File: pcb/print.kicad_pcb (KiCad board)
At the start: 2 copper layers, 12.4 x 46.4 mm, 23 parts, among them J1 USB_C_Receptacle_USB2.0_16P, J2 WS2812, SW1 Cycle, U1 FT232RL, U2 ATtiny85-20S

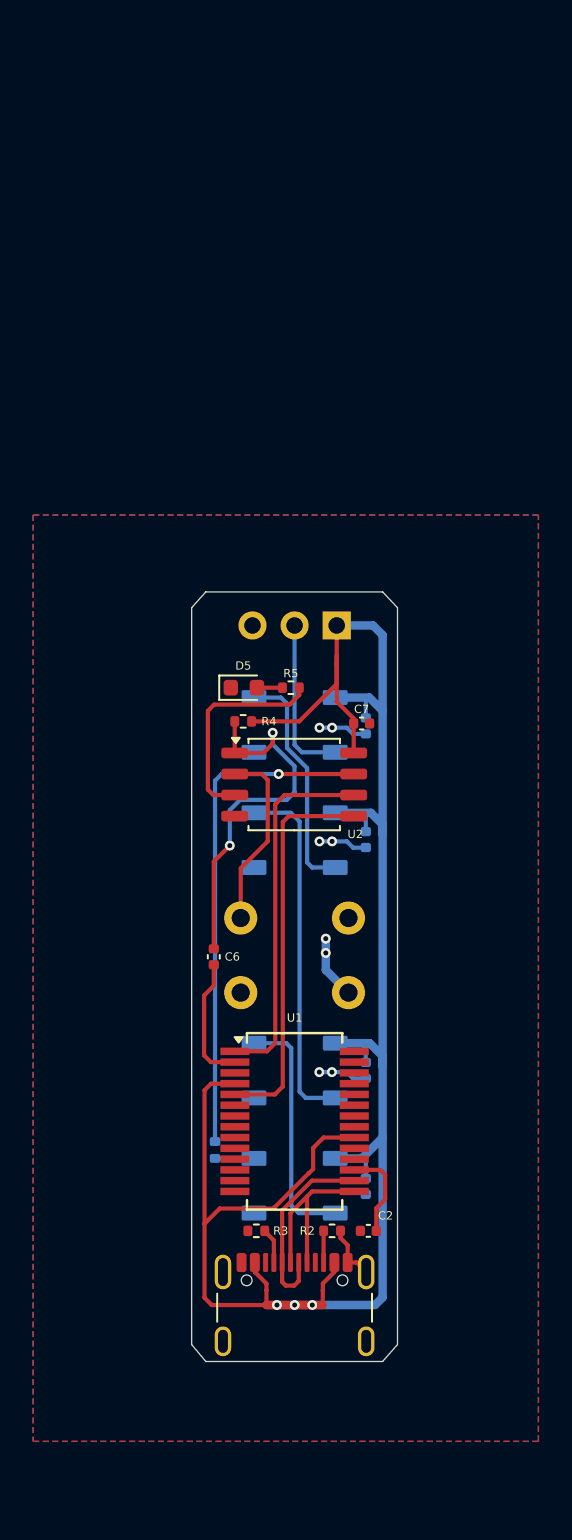
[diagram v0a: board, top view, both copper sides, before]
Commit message: pcb v1.1.0 update
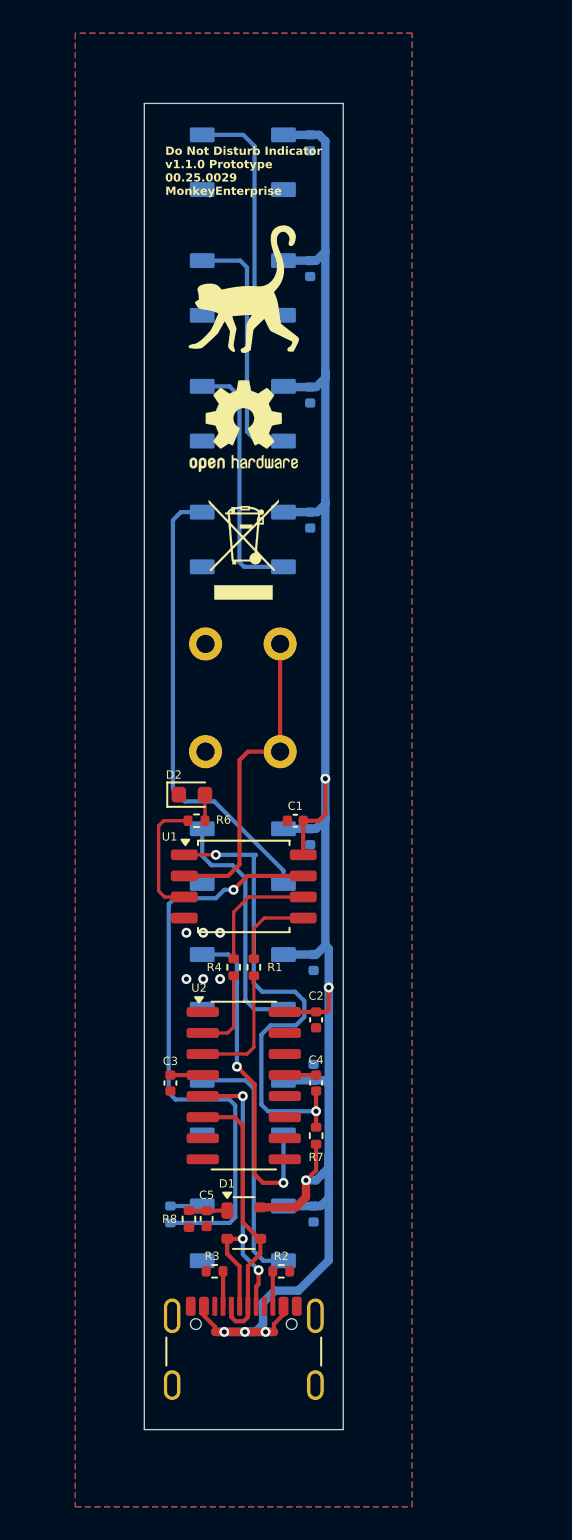
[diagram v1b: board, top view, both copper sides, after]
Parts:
- removed J2: WS2812, Connector_PinHeader_2.54mm:PinHeader_1x03_P2.54mm_Vertical
- added C10: 100nF, Capacitor_SMD:C_0402_1005Metric, B.Cu at (152.1, 74.0)
- added C11: 100nF, Capacitor_SMD:C_0402_1005Metric, B.Cu at (152.1, 66.4)
- added C12: 100nF, Capacitor_SMD:C_0402_1005Metric, B.Cu at (152.1, 58.8)
- added C13: 100nF, Capacitor_SMD:C_0402_1005Metric, B.Cu at (152.1, 51.2)
- added C8: 100nF, Capacitor_SMD:C_0402_1005Metric, B.Cu at (152.3, 100.7)
- added C9: 100nF, Capacitor_SMD:C_0402_1005Metric, B.Cu at (152.1, 93.1)
- added D10: WS2812B, Lib_WS2812B:LED_WS2812B_PLCC4_5.0x5.0mm_P3.2mm, B.Cu at (148.0, 52.4)
- added D6: WS2812B, Lib_WS2812B:LED_WS2812B_PLCC4_5.0x5.0mm_P3.2mm, B.Cu at (148.0, 94.2)
- added D7: WS2812B, Lib_WS2812B:LED_WS2812B_PLCC4_5.0x5.0mm_P3.2mm, B.Cu at (148.0, 75.1)
- added D8: WS2812B, Lib_WS2812B:LED_WS2812B_PLCC4_5.0x5.0mm_P3.2mm, B.Cu at (148.0, 67.5)
- added D9: WS2812B, Lib_WS2812B:LED_WS2812B_PLCC4_5.0x5.0mm_P3.2mm, B.Cu at (148.0, 60.0)
- added R6: 4K7, Resistor_SMD:R_0402_1005Metric, F.Cu at (145.2, 92.1)
- added R7: 10K0, Resistor_SMD:R_0402_1005Metric, F.Cu at (152.5, 111.1)
- added R8: 1M0, Resistor_SMD:R_0402_1005Metric, F.Cu at (144.8, 116.1)
- added REF**: WEEE-Logo_4.2x6mm_SilkScreen, Symbol:WEEE-Logo_4.2x6mm_SilkScreen, F.Cu at (148.1, 75.7)
- added REF**: OSHW-Logo2_7.3x6mm_SilkScreen, Symbol:OSHW-Logo2_7.3x6mm_SilkScreen, F.Cu at (148.1, 68.3)
- C1, C3, C4, G***: moved to F.Cu
- C5: value 100nF -> 4.7nF/1kV; moved to F.Cu
- C6, C7: moved to B.Cu
- D1: value WS2812B -> PRTR5V0U2X; footprint LED_SMD:LED_WS2812B_PLCC4_5.0x5.0mm_P3.2mm -> Package_TO_SOT_SMD:SOT-143; moved to F.Cu
- D2: value WS2812B -> CPU; footprint LED_SMD:LED_WS2812B_PLCC4_5.0x5.0mm_P3.2mm -> Diode_SMD:D_0603_1608Metric; moved to F.Cu
- D3, D4: footprint LED_SMD:LED_WS2812B_PLCC4_5.0x5.0mm_P3.2mm -> Lib_WS2812B:LED_WS2812B_PLCC4_5.0x5.0mm_P3.2mm
- D5: value CPU -> WS2812B; footprint Diode_SMD:D_0603_1608Metric -> Lib_WS2812B:LED_WS2812B_PLCC4_5.0x5.0mm_P3.2mm; moved to B.Cu
- R1: value 4K7 -> 1K0; moved to F.Cu
- R4: value 10K0 -> 1K0
- R5: value 4K7 -> 1K0; moved to B.Cu
- U1: value FT232RL -> ATtiny85-20S; footprint Package_SO:SSOP-28_5.3x10.2mm_P0.65mm -> Package_SO:SOIC-8_5.3x5.3mm_P1.27mm
- U2: value ATtiny85-20S -> CH340C; footprint Package_SO:SOIC-8_5.3x5.3mm_P1.27mm -> Package_SO:SOIC-16_3.9x9.9mm_P1.27mm
- moved G*** 60.7 mm to (148.1, 60.1), turned to 0 degrees
- moved R5 32.6 mm to (143.7, 115.9), turned to 90 degrees
- moved C5 31.2 mm to (145.8, 116.1)
- moved D3 23.9 mm to (148.0, 117.0)
- moved D4 23.3 mm to (148.0, 109.4)
- moved C1 22.5 mm to (151.2, 92.1), turned to 180 degrees
- moved C7 21.2 mm to (152.3, 107.3), turned to 90 degrees
- moved U2 18.4 mm to (148.1, 108.1)
- moved D2 17.8 mm to (145.0, 90.5), turned to 0 degrees
- moved D5 17.7 mm to (148.0, 101.8), turned to 180 degrees
- moved C6 16.6 mm to (152.3, 115.8), turned to -90 degrees
- moved C4 15.0 mm to (152.5, 107.9)
- moved R4 14.8 mm to (147.5, 100.9), turned to -90 degrees
- moved U1 14.5 mm to (148.1, 96.1)
- moved C2 13.1 mm to (152.5, 104.1), turned to -90 degrees
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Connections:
- C2 pad 1: +3.3V -> VBUS
- C3 pad 1: VBUS -> Net-(U2-V3)
- C4 pad 1: VBUS -> Net-(U2-~{DTR})
- C4 pad 2: GND -> /~{Reset} 
- C5 pad 1: VBUS -> Net-(D1-GND)
- C6 pad 1: Net-(U1-DTR) -> VBUS
- C6 pad 2: /~{Reset}  -> GND
- D1 pad 1: VBUS -> Net-(D1-GND)
- D1 pad 2: Net-(D1-DOUT) -> /USB_D_P
- D1 pad 3: GND -> /USB_D_N
- D1 pad 4: Net-(D1-DIN) -> VBUS
- D2 pad 1: VBUS -> GND
- D2 pad 2: Net-(D2-DOUT) -> Net-(D2-A)
- D3 pad 4: Net-(D2-DOUT) -> /LED_DATA_P
- D5 pad 1: GND -> VBUS
- D5 pad 2: Net-(D5-A) -> Net-(D5-DOUT)
- J1 pad A6: /USB_P -> /USB_D_P
- J1 pad A7: /USB_N -> /USB_D_N
- J1 pad B6: /USB_P -> /USB_D_P
- J1 pad B7: /USB_N -> /USB_D_N
- R1 pad 1: /LED_DATA_P -> Net-(U1-AREF/PB0)
- R1 pad 2: Net-(D1-DIN) -> /TX_D_P
- R4 pad 1: /~{Reset}  -> Net-(U1-PB1)
- R4 pad 2: VBUS -> /RX_D_P
- R5 pad 1: Net-(U2-XTAL2/PB4) -> Net-(U1-PB2)
- R5 pad 2: Net-(D5-A) -> /LED_DATA_P
- SW1 pad 1: Net-(U2-XTAL1/PB3) -> Net-(U1-XTAL1/PB3)
- U1 pad 1: /RX -> /~{Reset} 
- U1 pad 2: Net-(U1-DTR) -> Net-(U1-XTAL1/PB3)
- U1 pad 3: unconnected-(U1-RTS-Pad3) -> Net-(U1-XTAL2/PB4)
- U1 pad 4: VBUS -> GND
- U1 pad 5: /TX -> Net-(U1-AREF/PB0)
- U1 pad 6: unconnected-(U1-RI-Pad6) -> Net-(U1-PB1)
- U1 pad 7: GND -> Net-(U1-PB2)
- U1 pad 8: unconnected-(U1-NC-Pad8) -> VBUS
- U2 pad 1: /~{Reset}  -> GND
- U2 pad 2: Net-(U2-XTAL1/PB3) -> /RX_D_P
- U2 pad 3: Net-(U2-XTAL2/PB4) -> /TX_D_P
- U2 pad 4: GND -> Net-(U2-V3)
- U2 pad 5: /TX -> /USB_D_P
- U2 pad 6: /RX -> /USB_D_N
- U2 pad 7: /LED_DATA_P -> unconnected-(U2-NC-Pad7)
- U2 pad 8: VBUS -> unconnected-(U2-NC-Pad8)
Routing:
- net Net-(U1-PB2): track 0.00 -> 35.3 mm, vias 0 -> 1
- net /LED_DATA_P: track 30.3 -> 1.92 mm, vias 1 -> 0
- net Net-(D6-DOUT): track 0.00 -> 27.7 mm
- net /TX: track 23.5 -> 0.00 mm
- net /RX: track 22.0 -> 0.00 mm
- net Net-(D2-DOUT): track 21.6 -> 0.00 mm
- net /USB_D_P: track 0.00 -> 20.9 mm, vias 0 -> 3
- net Net-(U1-XTAL1/PB3): track 0.00 -> 19.1 mm
- net /USB_D_N: track 0.00 -> 16.8 mm
- net GND: track 16.1 -> 0.00 mm, vias 8 -> 6
- net Net-(D7-DOUT): track 0.00 -> 15.3 mm
- net Net-(D8-DOUT): track 0.00 -> 15.2 mm
- net Net-(D10-DIN): track 0.00 -> 15.1 mm
- net Net-(D5-DOUT): track 0.00 -> 14.8 mm
- net Net-(D1-DOUT): track 14.7 -> 0.00 mm
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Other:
- board size 12.4 x 46.4 mm -> 12 x 80 mm
- board text added: "${TITLE} ${REVISION} ${COMMENT2} ${COMMENT1} ${COMPANY}"
- board text removed: "DATA"
- board text removed: "GND"
- board text removed: "VCC"
